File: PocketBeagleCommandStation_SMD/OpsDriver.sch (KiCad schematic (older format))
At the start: 14 parts, among them U4 DRV8873HPWPR

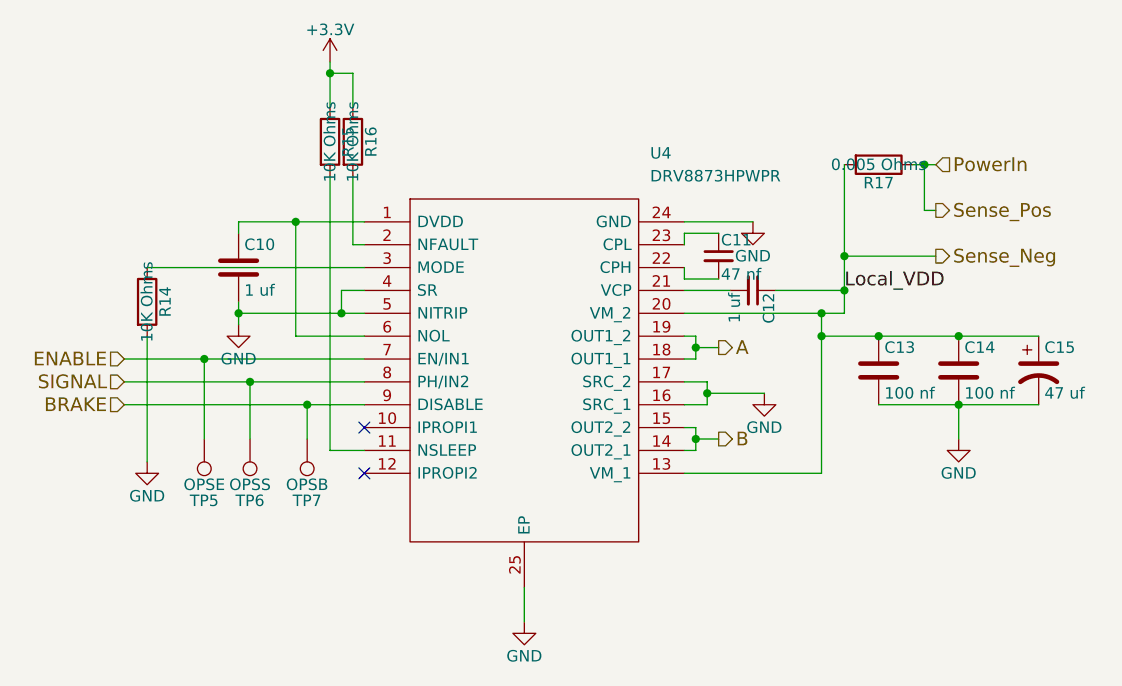
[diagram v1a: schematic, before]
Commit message: Continuing work on PocketBeagleCommandStation_SMD.
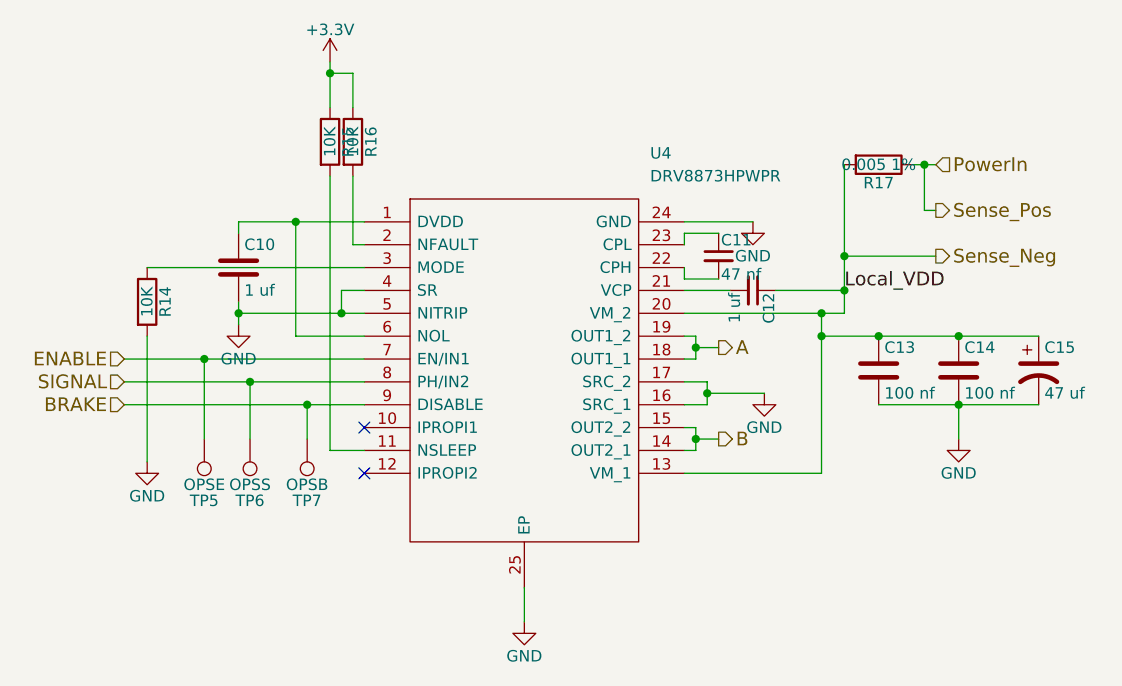
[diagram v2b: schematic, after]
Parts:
- R14, R16: value 10K Ohms -> 10K; footprint (none) -> Resistors_SMD:R_0603; Mouser Part Number (none) -> 279-CRGCQ0603F10K
- R15: value 10K Ohms -> 10K; footprint (none) -> Resistors_SMD:R_0603; Mouser Part Numer (none) -> 279-CRGCQ0603F10K
- R17: value 0.005 Ohms -> 0.005 1%; footprint (none) -> Resistors_SMD:R_0612; Mouser Part Number (none) -> 71-WSKW0612L5000FEA
- TP5, TP6, TP7: footprint (none) -> Measurement_Points:Measurement_Point_Round-SMD-Pad_Big
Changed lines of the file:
@@
 $EndComp
 $Comp
-L GND #PWR036
+L GND #PWR037
 U 1 1 6070432B
 P 5250 1800
-F 0 "#PWR036" H 5250 1550 50  0001 C CNN
+F 0 "#PWR037" H 5250 1550 50  0001 C CNN
 F 1 "GND" H 5250 1650 50  0000 C CNN
 F 2 "" H 5250 1800 50  0001 C CNN
@@
 $EndComp
 $Comp
-L GND #PWR037
+L GND #PWR038
 U 1 1 60704370
 P 4250 3550
-F 0 "#PWR037" H 4250 3300 50  0001 C CNN
+F 0 "#PWR038" H 4250 3300 50  0001 C CNN
 F 1 "GND" H 4250 3400 50  0000 C CNN
 F 2 "" H 4250 3550 50  0001 C CNN
@@
 P 5800 1550
 F 0 "R17" V 5880 1550 50  0000 C CNN
-F 1 "0.005 Ohms" V 5800 1550 50  0000 C CNN
-F 2 "" V 5730 1550 50  0001 C CNN
+F 1 "0.005 1%" V 5800 1550 50  0000 C CNN
+F 2 "Resistors_SMD:R_0612" V 5730 1550 50  0001 C CNN
 F 3 "" H 5800 1550 50  0001 C CNN
+F 4 "71-WSKW0612L5000FEA" V 5800 1550 60  0001 C CNN "Mouser Part Number"
 	1    5800 1550
 	0    1    1    0
@@
 $EndComp
 $Comp
-L GND #PWR038
+L GND #PWR039
 U 1 1 60704783
 P 6150 2750
-F 0 "#PWR038" H 6150 2500 50  0001 C CNN
+F 0 "#PWR039" H 6150 2500 50  0001 C CNN
 F 1 "GND" H 6150 2600 50  0000 C CNN
 F 2 "" H 6150 2750 50  0001 C CNN
@@
 $EndComp
 $Comp
-L GND #PWR039
+L GND #PWR040
 U 1 1 60704831
 P 5300 2550
-F 0 "#PWR039" H 5300 2300 50  0001 C CNN
+F 0 "#PWR040" H 5300 2300 50  0001 C CNN
 F 1 "GND" H 5300 2400 50  0000 C CNN
 F 2 "" H 5300 2550 50  0001 C CNN
@@
 $EndComp
 $Comp
-L GND #PWR040
+L GND #PWR041
 U 1 1 6070495B
 P 3000 2250
-F 0 "#PWR040" H 3000 2000 50  0001 C CNN
+F 0 "#PWR041" H 3000 2000 50  0001 C CNN
 F 1 "GND" H 3000 2100 50  0000 C CNN
 F 2 "" H 3000 2250 50  0001 C CNN
@@
 P 3500 1450
 F 0 "R16" V 3580 1450 50  0000 C CNN
-F 1 "10K Ohms" V 3500 1450 50  0000 C CNN
-F 2 "" V 3430 1450 50  0001 C CNN
+F 1 "10K" V 3500 1450 50  0000 C CNN
+F 2 "Resistors_SMD:R_0603" V 3430 1450 50  0001 C CNN
 F 3 "" H 3500 1450 50  0001 C CNN
+F 4 "279-CRGCQ0603F10K" V 3500 1450 60  0001 C CNN "Mouser Part Number"
 	1    3500 1450
 	1    0    0    -1
@@
 P 3400 1450
 F 0 "R15" V 3480 1450 50  0000 C CNN
-F 1 "10K Ohms" V 3400 1450 50  0000 C CNN
-F 2 "" V 3330 1450 50  0001 C CNN
+F 1 "10K" V 3400 1450 50  0000 C CNN
+F 2 "Resistors_SMD:R_0603" V 3330 1450 50  0001 C CNN
 F 3 "" H 3400 1450 50  0001 C CNN
+F 4 "279-CRGCQ0603F10K" V 3400 1450 60  0001 C CNN "Mouser Part Numer"
 	1    3400 1450
 	1    0    0    -1
 $EndComp
 $Comp
-L +3.3V #PWR041
+L +3.3V #PWR042
 U 1 1 60707495
 P 3400 1100
-F 0 "#PWR041" H 3400 950 50  0001 C CNN
+F 0 "#PWR042" H 3400 950 50  0001 C CNN
 F 1 "+3.3V" H 3400 1240 50  0000 C CNN
 F 2 "" H 3400 1100 50  0001 C CNN
@@
 P 2600 2150
 F 0 "R14" V 2680 2150 50  0000 C CNN
-F 1 "10K Ohms" V 2600 2150 50  0000 C CNN
-F 2 "" V 2530 2150 50  0001 C CNN
+F 1 "10K" V 2600 2150 50  0000 C CNN
+F 2 "Resistors_SMD:R_0603" V 2530 2150 50  0001 C CNN
 F 3 "" H 2600 2150 50  0001 C CNN
+F 4 "279-CRGCQ0603F10K" V 2600 2150 60  0001 C CNN "Mouser Part Number"
 	1    2600 2150
 	1    0    0    -1
 $EndComp
 $Comp
-L GND #PWR042
+L GND #PWR043
 U 1 1 607075FE
 P 2600 2850
-F 0 "#PWR042" H 2600 2600 50  0001 C CNN
+F 0 "#PWR043" H 2600 2600 50  0001 C CNN
 F 1 "GND" H 2600 2700 50  0000 C CNN
 F 2 "" H 2600 2850 50  0001 C CNN
@@
 F 0 "TP7" H 3300 3020 50  0000 C CNN
 F 1 "OPSB" H 3300 2950 50  0000 C CNN
-F 2 "" H 3500 2750 50  0001 C CNN
+F 2 "Measurement_Points:Measurement_Point_Round-SMD-Pad_Big" H 3500 2750 50  0001 C CNN
 F 3 "" H 3500 2750 50  0001 C CNN
 	1    3300 2750
@@
 F 0 "TP6" H 3050 3020 50  0000 C CNN
 F 1 "OPSS" H 3050 2950 50  0000 C CNN
-F 2 "" H 3250 2750 50  0001 C CNN
+F 2 "Measurement_Points:Measurement_Point_Round-SMD-Pad_Big" H 3250 2750 50  0001 C CNN
 F 3 "" H 3250 2750 50  0001 C CNN
 	1    3050 2750
@@
 F 0 "TP5" H 2850 3020 50  0000 C CNN
 F 1 "OPSE" H 2850 2950 50  0000 C CNN
-F 2 "" H 3050 2750 50  0001 C CNN
+F 2 "Measurement_Points:Measurement_Point_Round-SMD-Pad_Big" H 3050 2750 50  0001 C CNN
 F 3 "" H 3050 2750 50  0001 C CNN
 	1    2850 2750
